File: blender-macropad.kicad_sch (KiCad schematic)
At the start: 29 parts, among them J1 Conn_02x12_Counter_Clockwise, J2 Conn_01x07, SW1 SW_Push, SW10 SW_Push, SW11 SW_Push, SW12 SW_Push, SW13 RotaryEncoder_Switch, SW2 SW_Push, SW3 SW_Push, SW4 SW_Push, SW5 SW_Push, SW6 SW_Push, SW7 SW_Push, SW8 SW_Push, SW9 SW_Push

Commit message: initial pcb layout attempt
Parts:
- J1: footprint (none) -> Connector_PinHeader_2.54mm:PinHeader_2x12_P2.54mm_Vertical
- J2: footprint (none) -> Connector_PinHeader_2.54mm:PinHeader_1x07_P2.54mm_Vertical
- R1, R2: footprint (none) -> Resistor_SMD:R_0805_2012Metric
- SW13: footprint (none) -> Rotary_Encoder:RotaryEncoder_Alps_EC11E-Switch_Vertical_H20mm
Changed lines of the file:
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@@
 			)
 		)
-		(property "Footprint" ""
+		(property "Footprint" "Resistor_SMD:R_0805_2012Metric"
 			(at 118.872 76.2 90)
 			(hide yes)
@@
 			)
 		)
-		(property "Footprint" ""
+		(property "Footprint" "Connector_PinHeader_2.54mm:PinHeader_2x12_P2.54mm_Vertical"
 			(at 110.49 101.6 0)
 			(hide yes)
@@
 			)
 		)
-		(property "Footprint" ""
+		(property "Footprint" "Connector_PinHeader_2.54mm:PinHeader_1x07_P2.54mm_Vertical"
 			(at 140.97 59.69 0)
 			(hide yes)
@@
 			)
 		)
-		(property "Footprint" ""
+		(property "Footprint" "Resistor_SMD:R_0805_2012Metric"
 			(at 109.982 76.2 90)
 			(hide yes)
@@
 			)
 		)
-		(property "Footprint" ""
+		(property "Footprint" "Rotary_Encoder:RotaryEncoder_Alps_EC11E-Switch_Vertical_H20mm"
 			(at 113.03 59.436 0)
 			(hide yes)

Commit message: reworked pcb layout
polished pc layout with correct dimension
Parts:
- SW1, SW10, SW11, SW12, SW2, SW3, SW4, SW5, SW6, SW7, SW8, SW9: footprint Button_Switch_SMD:Nidec_Copal_CAS-120A -> Button_Switch_Keyboard:SW_Cherry_MX_1.00u_PCB
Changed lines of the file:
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@@
 			)
 		)
-		(property "Footprint" "Button_Switch_SMD:Nidec_Copal_CAS-120A"
+		(property "Footprint" "Button_Switch_Keyboard:SW_Cherry_MX_1.00u_PCB"
 			(at 135.89 97.79 0)
 			(hide yes)
@@
 			)
 		)
-		(property "Footprint" "Button_Switch_SMD:Nidec_Copal_CAS-120A"
+		(property "Footprint" "Button_Switch_Keyboard:SW_Cherry_MX_1.00u_PCB"
 			(at 166.37 97.79 0)
 			(hide yes)
@@
 			)
 		)
-		(property "Footprint" "Button_Switch_SMD:Nidec_Copal_CAS-120A"
+		(property "Footprint" "Button_Switch_Keyboard:SW_Cherry_MX_1.00u_PCB"
 			(at 135.89 76.2 0)
 			(hide yes)
@@
 			)
 		)
-		(property "Footprint" "Button_Switch_SMD:Nidec_Copal_CAS-120A"
+		(property "Footprint" "Button_Switch_Keyboard:SW_Cherry_MX_1.00u_PCB"
 			(at 151.13 76.2 0)
 			(hide yes)
@@
 			)
 		)
-		(property "Footprint" "Button_Switch_SMD:Nidec_Copal_CAS-120A"
+		(property "Footprint" "Button_Switch_Keyboard:SW_Cherry_MX_1.00u_PCB"
 			(at 151.13 97.79 0)
 			(hide yes)
@@
 			)
 		)
-		(property "Footprint" "Button_Switch_SMD:Nidec_Copal_CAS-120A"
+		(property "Footprint" "Button_Switch_Keyboard:SW_Cherry_MX_1.00u_PCB"
 			(at 135.89 119.38 0)
 			(hide yes)
@@
 			)
 		)
-		(property "Footprint" "Button_Switch_SMD:Nidec_Copal_CAS-120A"
+		(property "Footprint" "Button_Switch_Keyboard:SW_Cherry_MX_1.00u_PCB"
 			(at 166.37 119.38 0)
 			(hide yes)
@@
 			)
 		)
-		(property "Footprint" "Button_Switch_SMD:Nidec_Copal_CAS-120A"
+		(property "Footprint" "Button_Switch_Keyboard:SW_Cherry_MX_1.00u_PCB"
 			(at 181.61 76.2 0)
 			(hide yes)
@@
 			)
 		)
-		(property "Footprint" "Button_Switch_SMD:Nidec_Copal_CAS-120A"
+		(property "Footprint" "Button_Switch_Keyboard:SW_Cherry_MX_1.00u_PCB"
 			(at 151.13 119.38 0)
 			(hide yes)
@@
 			)
 		)
-		(property "Footprint" "Button_Switch_SMD:Nidec_Copal_CAS-120A"
+		(property "Footprint" "Button_Switch_Keyboard:SW_Cherry_MX_1.00u_PCB"
 			(at 166.37 76.2 0)
 			(hide yes)
@@
 			)
 		)
-		(property "Footprint" "Button_Switch_SMD:Nidec_Copal_CAS-120A"
+		(property "Footprint" "Button_Switch_Keyboard:SW_Cherry_MX_1.00u_PCB"
 			(at 181.61 97.79 0)
 			(hide yes)
@@
 			)
 		)
-		(property "Footprint" "Button_Switch_SMD:Nidec_Copal_CAS-120A"
+		(property "Footprint" "Button_Switch_Keyboard:SW_Cherry_MX_1.00u_PCB"
 			(at 181.61 119.38 0)
 			(hide yes)

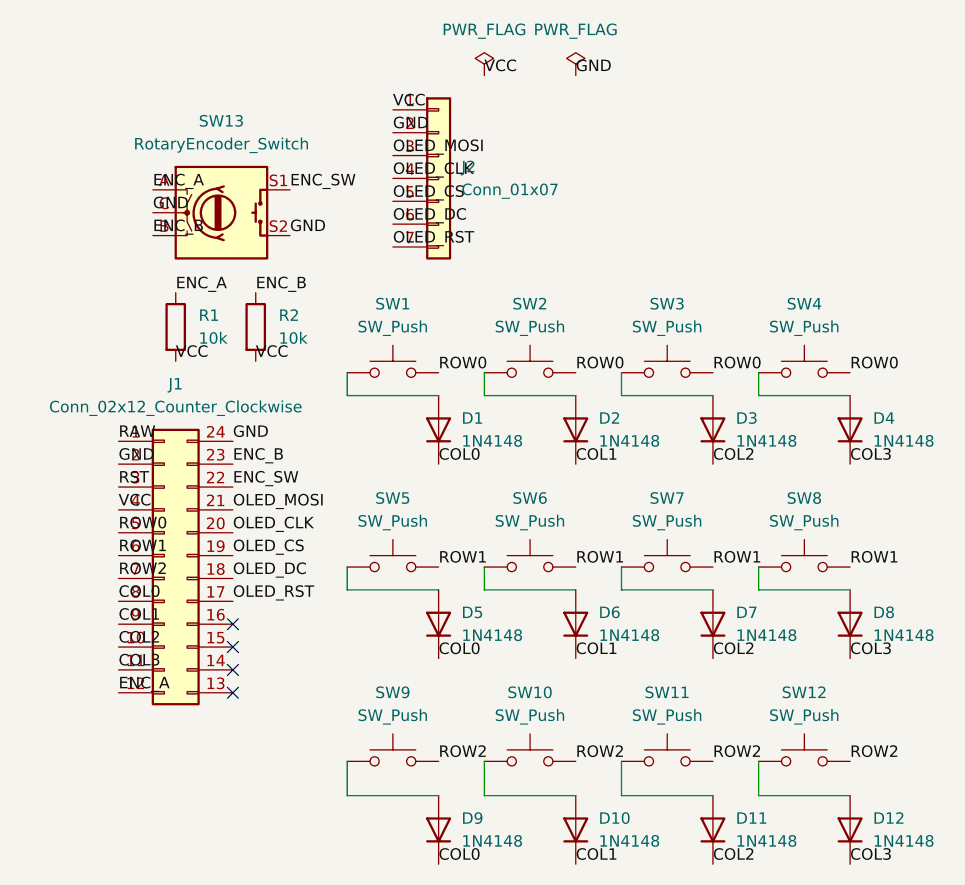
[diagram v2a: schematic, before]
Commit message: Updated PCB
Fixed PCB
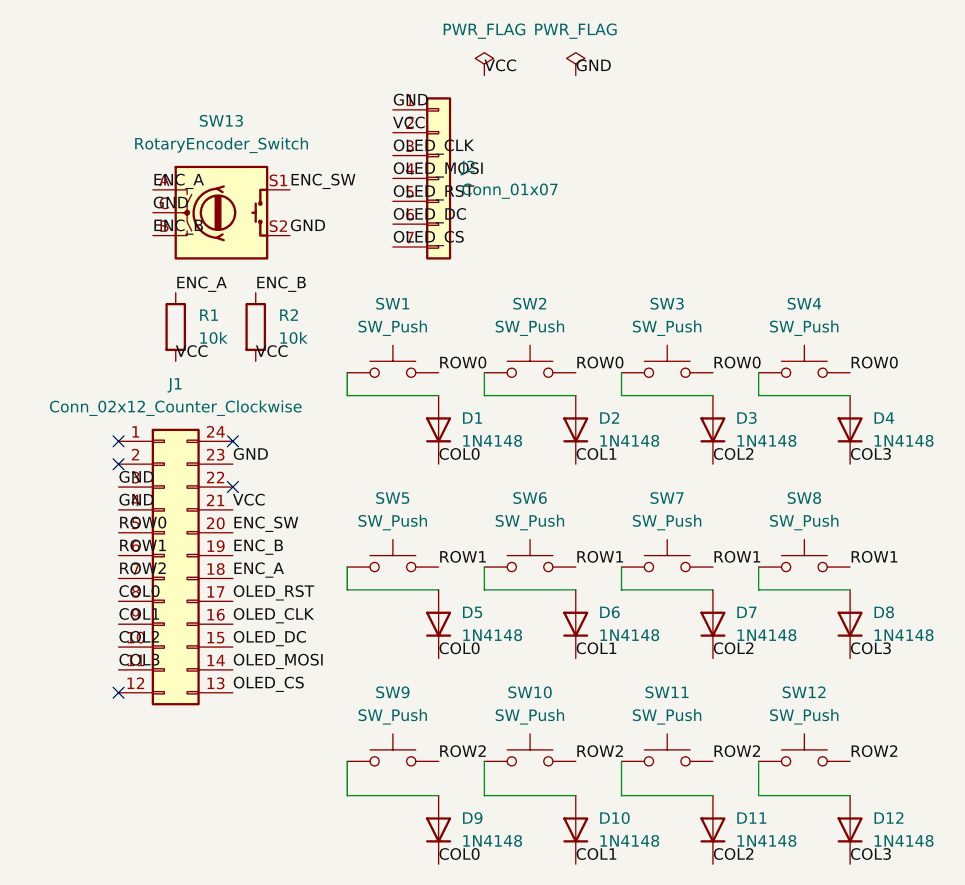
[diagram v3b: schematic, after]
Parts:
- J1: footprint Connector_PinHeader_2.54mm:PinHeader_2x12_P2.54mm_Vertical -> Package_DIP:DIP-24_W15.24mm
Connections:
- net RST is gone; now on net GND: J1.3 (Pin_3)
- net ENC_A: now also J1.18 (Pin_18); no longer J1.12 (Pin_12)
- net ENC_B: now also J1.19 (Pin_19); no longer J1.23 (Pin_23)
- net ENC_SW: now also J1.20 (Pin_20); no longer J1.22 (Pin_22)
- net GND: now also J1.23 (Pin_23), J1.4 (Pin_4), J2.1 (Pin_1); no longer J1.2 (Pin_2), J1.24 (Pin_24), J2.2 (Pin_2)
- net OLED_CLK: now also J1.16 (Pin_16), J2.3 (Pin_3); no longer J1.20 (Pin_20), J2.4 (Pin_4)
- net OLED_CS: now also J1.13 (Pin_13), J2.7 (Pin_7); no longer J1.19 (Pin_19), J2.5 (Pin_5)
- net OLED_DC: now also J1.15 (Pin_15); no longer J1.18 (Pin_18)
- net OLED_MOSI: now also J1.14 (Pin_14), J2.4 (Pin_4); no longer J1.21 (Pin_21), J2.3 (Pin_3)
- net OLED_RST: now also J2.5 (Pin_5); no longer J2.7 (Pin_7)
- net VCC: now also J1.21 (Pin_21), J2.2 (Pin_2); no longer J1.4 (Pin_4), J2.1 (Pin_1)
- net RAW: no longer names the net of J1.1 (Pin_1)
- no-connect marks 4 -> 5
